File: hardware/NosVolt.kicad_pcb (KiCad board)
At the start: 2 copper layers, 100 x 60 mm, 119 parts, among them CN201 100nF, J101 INPUTS, J102 OUTPUTS, J201 BAT_SENSE, J202 BAT_NTC, J401 USB_C_Receptacle_USB2.0_16P, Q1101 2N7002, Q1102 AO4407A, Q801 2N7002, Q802 AO4407A, Q901 2N7002, Q902 AO4407A, SW101 SW_Reset, SW102 SSSS811101, U1001 INA226, U101 GMT028-05, U102 ESP32-S3-WROOM-1, U1201 INA226, U201 ADS1115IDGS, U301 MP2307DN-LF-Z, U401 AP7361-33ER-13, U402 USBLC6-2SC6, U501 INA226, U601 INA226, U701 INA226

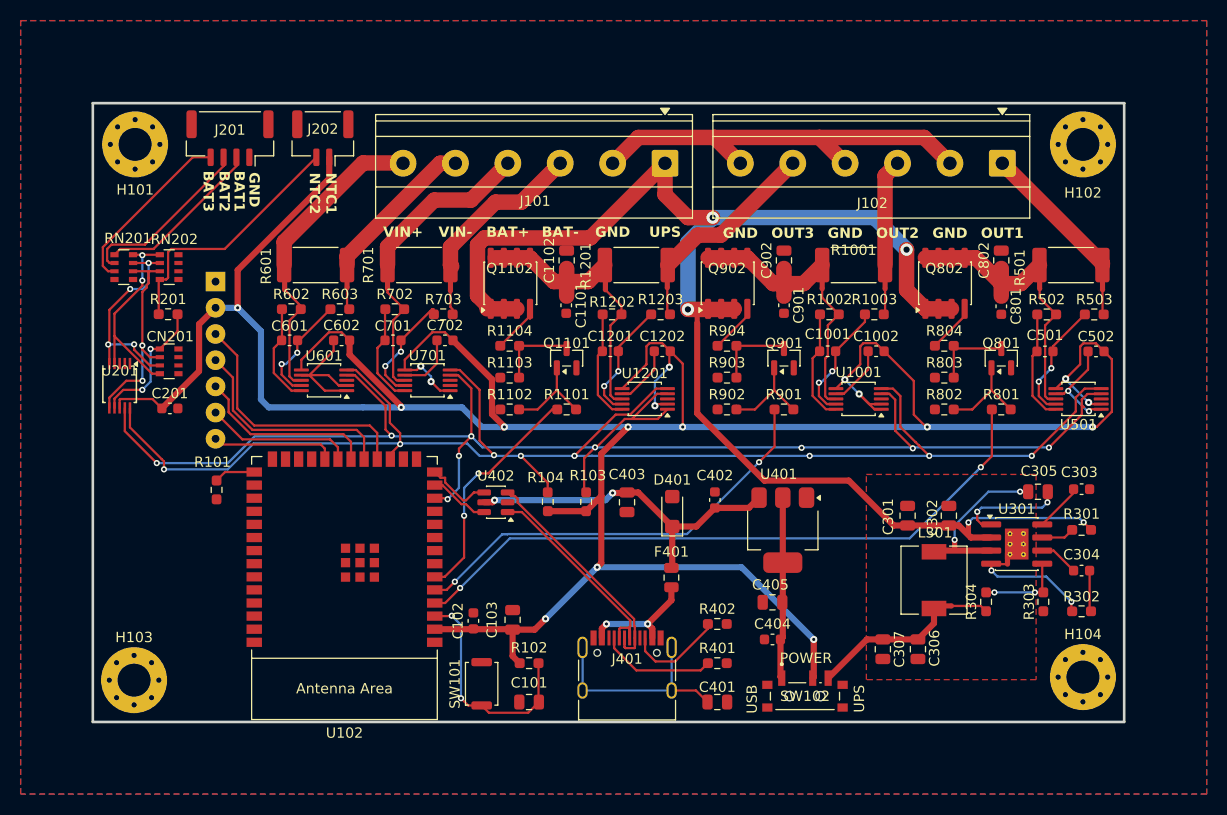
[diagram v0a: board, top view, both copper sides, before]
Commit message: fix errors
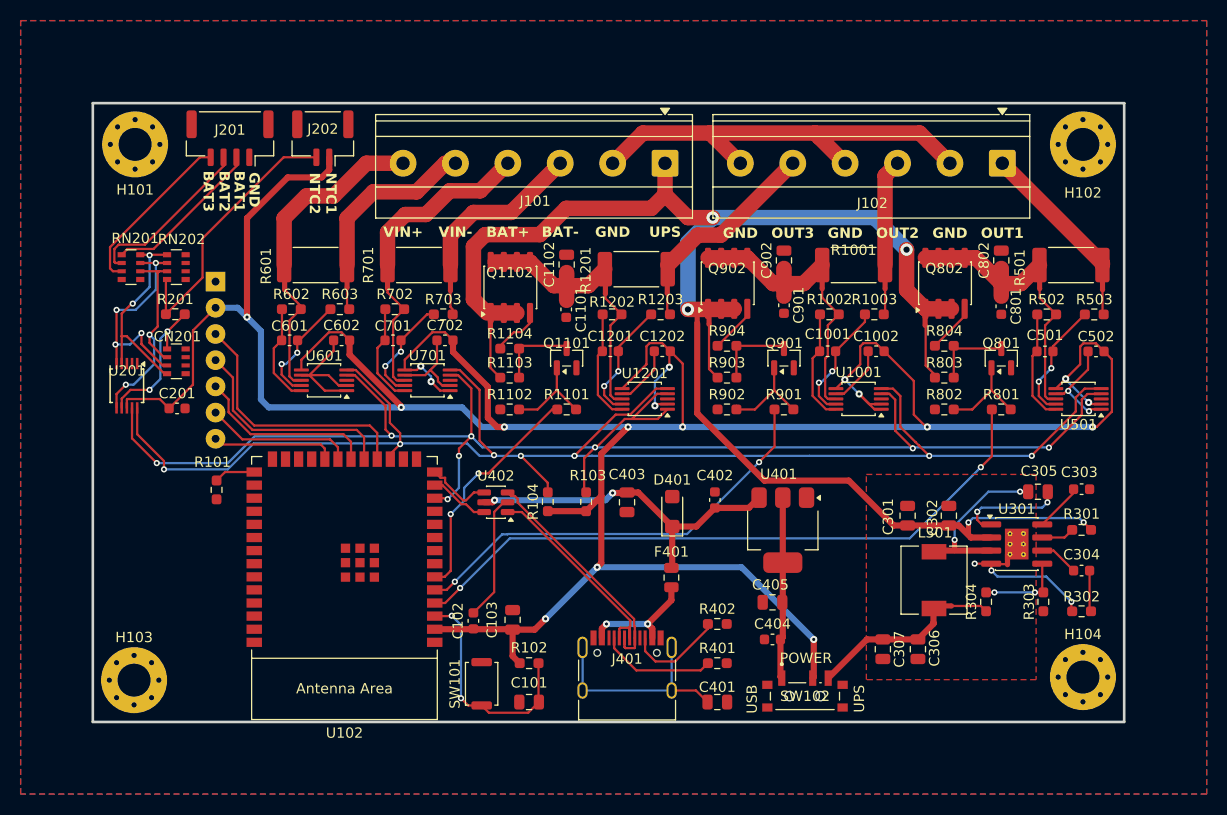
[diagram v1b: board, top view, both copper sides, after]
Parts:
- added NT1101: NetTie_2, NetTie:NetTie-2_SMD_Pad0.5mm, F.Cu at (141.2, 59.2)
- added NT801: NetTie_2, NetTie:NetTie-2_SMD_Pad0.5mm, F.Cu at (183.4, 58.9)
- added NT901: NetTie_2, NetTie:NetTie-2_SMD_Pad0.5mm, F.Cu at (162.4, 58.8)
- NT301: value NetTie_SW_BS -> NetTie_IN_EN
- NT302: value NetTie_SW_FB -> NetTie_GND
- NT303: value NetTie_IN_EN -> NetTie_SW_BS
- NT304: value NetTie_GND -> NetTie_SW_FB
- moved NT304 7.47 mm to (185.5, 86.5), turned to 180 degrees
- moved NT302 7.44 mm to (191.4, 82.0), turned to 90 degrees
- moved NT303 2.17 mm to (186.2, 80.7), turned to -90 degrees
- moved NT301 2.12 mm to (187.6, 79.0), turned to 90 degrees
- moved C201 0.70 mm to (110.9, 67.4)
- moved CN201 0.70 mm to (110.8, 62.8)
- moved R201 0.70 mm to (110.7, 58.3)
- moved RN201 0.70 mm to (106.4, 53.7)
- moved RN202 0.70 mm to (110.8, 53.7)
- moved U201 0.70 mm to (106.0, 65.2)
- moved NT1202 0.55 mm to (158.4, 55.8)
- moved C1102 0.40 mm to (148.6, 53.5)
- moved C1101 0.40 mm to (148.6, 57.8)
- moved NT1201 0.40 mm to (152.4, 55.8)
- moved Q1102 0.40 mm to (143.2, 55.7)
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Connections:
- NT301 pad 1: Net-(C305-Pad2) -> /+12V_UPS
- NT301 pad 2: /MP2307/SW -> Net-(NT301-Pad2)
- NT302 pad 1: Net-(NT302-Pad1) -> GND
- NT302 pad 2: +3V3_UPS -> /MP2307/PWR_GND
- NT303 pad 1: /+12V_UPS -> Net-(C305-Pad2)
- NT303 pad 2: Net-(NT303-Pad2) -> /MP2307/SW
- NT304 pad 1: GND -> Net-(NT304-Pad1)
- NT304 pad 2: /MP2307/PWR_GND -> +3V3_UPS
- R301 pad 1: Net-(NT303-Pad2) -> Net-(NT301-Pad2)
- R304 pad 2: Net-(NT302-Pad1) -> Net-(NT304-Pad1)
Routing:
- net GND: track 54.0 -> 70.9 mm, vias 4 -> 5
- net Net-(NT303-Pad2): track 12.5 -> 0.00 mm, vias 2 -> 0
- net Net-(NT301-Pad2): track 0.00 -> 12.5 mm, vias 0 -> 2
- net Net-(NT801-Pad1): track 0.00 -> 5.63 mm
- net Net-(NT901-Pad1): track 0.00 -> 5.51 mm
- net Net-(NT1101-Pad1): track 0.00 -> 5.18 mm
- net Net-(NT304-Pad1): track 0.00 -> 3.56 mm
- net Net-(NT302-Pad1): track 3.56 -> 0.00 mm
- net +3V3: track 306.5 -> 309.1 mm
- net /SHUNT_IN_LO: track 15.1 -> 17.3 mm
- net Net-(RN201-R2.2): track 20.8 -> 22.4 mm
- net Net-(J202-Pin_2): track 25.0 -> 26.5 mm
- net /SHUNT_OUT_HI: track 41.8 -> 43.4 mm
- net /SHUNT_IN_HI: track 17.0 -> 18.3 mm
- net Net-(U201-AIN3): track 13.3 -> 14.4 mm
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
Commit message: fix errors 2
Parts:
- NT301: value NetTie_IN_EN -> NetTie_SW_BS
- NT302: value NetTie_GND -> NetTie_SW_FB
- NT303: value NetTie_SW_BS -> NetTie_IN_EN
- NT304: value NetTie_SW_FB -> NetTie_GND
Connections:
- NT301 pad 1: /+12V_UPS -> Net-(C305-Pad2)
- NT301 pad 2: Net-(NT301-Pad2) -> /MP2307/SW
- NT302 pad 1: GND -> Net-(NT302-Pad1)
- NT302 pad 2: /MP2307/PWR_GND -> +3V3_UPS
- NT303 pad 1: Net-(C305-Pad2) -> /+12V_UPS
- NT303 pad 2: /MP2307/SW -> Net-(NT303-Pad2)
- NT304 pad 1: Net-(NT304-Pad1) -> GND
- NT304 pad 2: +3V3_UPS -> /MP2307/PWR_GND
- R301 pad 1: Net-(NT301-Pad2) -> Net-(NT303-Pad2)
- R304 pad 2: Net-(NT304-Pad1) -> Net-(NT302-Pad1)
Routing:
- net Net-(NT301-Pad2): track 12.5 -> 0.00 mm, vias 2 -> 0
- net /MP2307/SW: track 5.59 -> 18.1 mm, vias 0 -> 2
- net GND: track 70.9 -> 74.4 mm
- net Net-(NT304-Pad1): track 3.56 -> 0.00 mm
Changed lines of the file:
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@@
 	(net 92 "unconnected-(U102-GPIO1{slash}TOUCH1{slash}ADC1_CH0-Pad39)")
 	(net 93 "unconnected-(U102-GPIO38{slash}FSPIWP{slash}SUBSPIWP-Pad31)")
-	(net 94 "Net-(NT301-Pad2)")
+	(net 94 "Net-(NT302-Pad1)")
 	(net 95 "/MP2307/PWR_GND")
 	(net 96 "Net-(NT901-Pad1)")
@@
 	(net 118 "Net-(U1201-Vbus)")
 	(net 119 "Net-(NT1202-Pad2)")
-	(net 120 "Net-(NT304-Pad1)")
+	(net 120 "Net-(NT303-Pad2)")
 	(net 121 "Net-(NT801-Pad1)")
 	(net 122 "Net-(NT1101-Pad1)")
@@
 			)
 		)
-		(property "Value" "NetTie_GND"
+		(property "Value" "NetTie_SW_FB"
 			(at 0 1.2 90)
 			(layer "F.Fab")
@@
 			(size 0.5 0.5)
 			(layers "F.Cu")
-			(net 27 "GND")
+			(net 94 "Net-(NT302-Pad1)")
 			(pinfunction "1")
 			(pintype "passive")
@@
 			(size 0.5 0.5)
 			(layers "F.Cu")
-			(net 95 "/MP2307/PWR_GND")
+			(net 58 "+3V3_UPS")
 			(pinfunction "2")
 			(pintype "passive")
@@
 			(layers "F.Cu" "F.Mask" "F.Paste")
 			(roundrect_rratio 0.25)
-			(net 94 "Net-(NT301-Pad2)")
+			(net 120 "Net-(NT303-Pad2)")
 			(pintype "passive")
 		)
@@
 			)
 		)
-		(property "Value" "NetTie_SW_BS"
+		(property "Value" "NetTie_IN_EN"
 			(at 0 1.2 90)
 			(layer "F.Fab")
@@
 			(size 0.5 0.5)
 			(layers "F.Cu")
-			(net 113 "Net-(C305-Pad2)")
+			(net 63 "/+12V_UPS")
 			(pinfunction "1")
 			(pintype "passive")
@@
 			(size 0.5 0.5)
 			(layers "F.Cu")
-			(net 64 "/MP2307/SW")
+			(net 120 "Net-(NT303-Pad2)")
 			(pinfunction "2")
 			(pintype "passive")
@@
 			)
 		)
-		(property "Value" "NetTie_IN_EN"
+		(property "Value" "NetTie_SW_BS"
 			(at 0 1.2 90)
 			(layer "F.Fab")
@@
 			(size 0.5 0.5)
 			(layers "F.Cu")
-			(net 63 "/+12V_UPS")
+			(net 113 "Net-(C305-Pad2)")
 			(pinfunction "1")
 			(pintype "passive")
@@
 			(size 0.5 0.5)
 			(layers "F.Cu")
-			(net 94 "Net-(NT301-Pad2)")
+			(net 64 "/MP2307/SW")
 			(pinfunction "2")
 			(pintype "passive")
@@
 			(layers "F.Cu" "F.Mask" "F.Paste")
 			(roundrect_rratio 0.25)
-			(net 120 "Net-(NT304-Pad1)")
+			(net 94 "Net-(NT302-Pad1)")
 			(pintype "passive")
 		)
@@
 			)
 		)
-		(property "Value" "NetTie_SW_FB"
+		(property "Value" "NetTie_GND"
 			(at 0 1.2 0)
 			(layer "F.Fab")
@@
 			(size 0.5 0.5)
 			(layers "F.Cu")
-			(net 120 "Net-(NT304-Pad1)")
+			(net 27 "GND")
 			(pinfunction "1")
 			(pintype "passive")
@@
 			(size 0.5 0.5)
 			(layers "F.Cu")
-			(net 58 "+3V3_UPS")
+			(net 95 "/MP2307/PWR_GND")
 			(pinfunction "2")
 			(pintype "passive")
@@
 	)
 	(segment
+		(start 185.96 86.55)
+		(end 188.7975 86.55)
+		(width 0.22)
+		(layer "F.Cu")
+		(net 27)
+	)
+	(segment
+		(start 188.7975 86.55)
+		(end 189.31 87.0625)
+		(width 0.22)
+		(layer "F.Cu")
+		(net 27)
+	)
+	(segment
 		(start 142.9175 76.5)
 		(end 142.54889 76.5)
@@
 	)
 	(segment
+		(start 199.4825 79.176667)
+		(end 199.4825 79.1625)
+		(width 0.22)
+		(layer "F.Cu")
+		(net 64)
+	)
+	(segment
 		(start 184.375 81.185)
 		(end 184.26 81.3)
@@
 	)
 	(segment
+		(start 199.4825 79.1625)
+		(end 198.77 78.45)
+		(width 0.22)
+		(layer "F.Cu")
+		(net 64)
+	)
+	(segment
 		(start 189.805 81.185)
 		(end 184.375 81.185)
@@
 		(net 64)
 	)
+	(via
+		(at 198.77 78.45)
+		(size 0.6)
+		(drill 0.3)
+		(layers "F.Cu" "B.Cu")
+		(net 64)
+	)
+	(via
+		(at 187.6 78.455508)
+		(size 0.6)
+		(drill 0.3)
+		(layers "F.Cu" "B.Cu")
+		(net 64)
+	)
+	(segment
+		(start 198.35 78.03)
+		(end 188.025508 78.03)
+		(width 0.22)
+		(layer "B.Cu")
+		(net 64)
+	)
+	(segment
+		(start 188.025508 78.03)
+		(end 187.6 78.455508)
+		(width 0.22)
+		(layer "B.Cu")
+		(net 64)
+	)
+	(segment
+		(start 198.77 78.45)
+		(end 198.35 78.03)
+		(width 0.22)
+		(layer "B.Cu")
+		(net 64)
+	)
 	(segment
 		(start 139.6 51.7)
@@
 	)
 	(segment
-		(start 199.4825 79.176667)
-		(end 199.4825 79.1625)
-		(width 0.22)
-		(layer "F.Cu")
-		(net 94)
-	)
-	(segment
-		(start 199.4825 79.1625)
-		(end 198.77 78.45)
-		(width 0.22)
-		(layer "F.Cu")
-		(net 94)
-	)
-	(via
-		(at 198.77 78.45)
-		(size 0.6)
-		(drill 0.3)
-		(layers "F.Cu" "B.Cu")
-		(net 94)
-	)
-	(via
-		(at 187.6 78.455508)
-		(size 0.6)
-		(drill 0.3)
-		(layers "F.Cu" "B.Cu")
-		(net 94)
-	)
-	(segment
-		(start 198.35 78.03)
-		(end 188.025508 78.03)
-		(width 0.22)
-		(layer "B.Cu")
-		(net 94)
-	)
-	(segment
-		(start 188.025508 78.03)
-		(end 187.6 78.455508)
-		(width 0.22)
-		(layer "B.Cu")
-		(net 94)
-	)
-	(segment
-		(start 198.77 78.45)
-		(end 198.35 78.03)
-		(width 0.22)
-		(layer "B.Cu")
-		(net 94)
-	)
-	(segment
 		(start 162.45 59.25)
 		(end 162.45 63.587333)
@@
 	)
 	(segment
-		(start 185.96 86.55)
-		(end 188.7975 86.55)
-		(width 0.22)
-		(layer "F.Cu")
-		(net 120)
-	)
-	(segment
-		(start 188.7975 86.55)
-		(end 189.31 87.0625)
-		(width 0.22)
-		(layer "F.Cu")
-		(net 120)
-	)
-	(segment
